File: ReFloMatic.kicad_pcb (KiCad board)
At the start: 2 copper layers, 54.4 x 85.3 mm, 150 parts, among them CON2 MicroSD_Card, P1 PROG, P2 THERMOCOUPLE, P3 DOOR_SERVO, P4 OVEN, P5 USB_B, P6 PWR_CONN, Q1 MMUN2211, Q2 MMUN2111, Q3 MMUN2111, Q4 MMUN2211, U1 STM32F030C, U2 MAX31855KASA

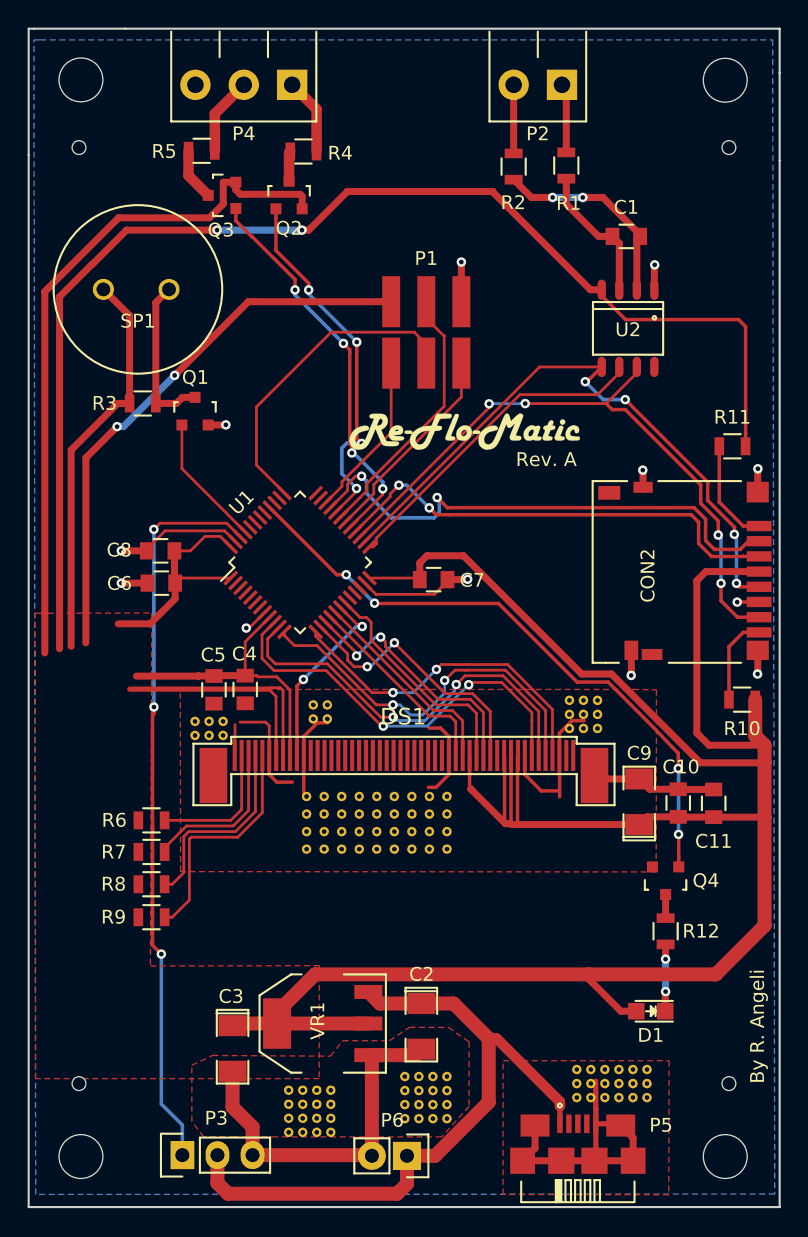
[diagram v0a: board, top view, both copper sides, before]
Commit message: Finished PCB layout. Generated gerbers.
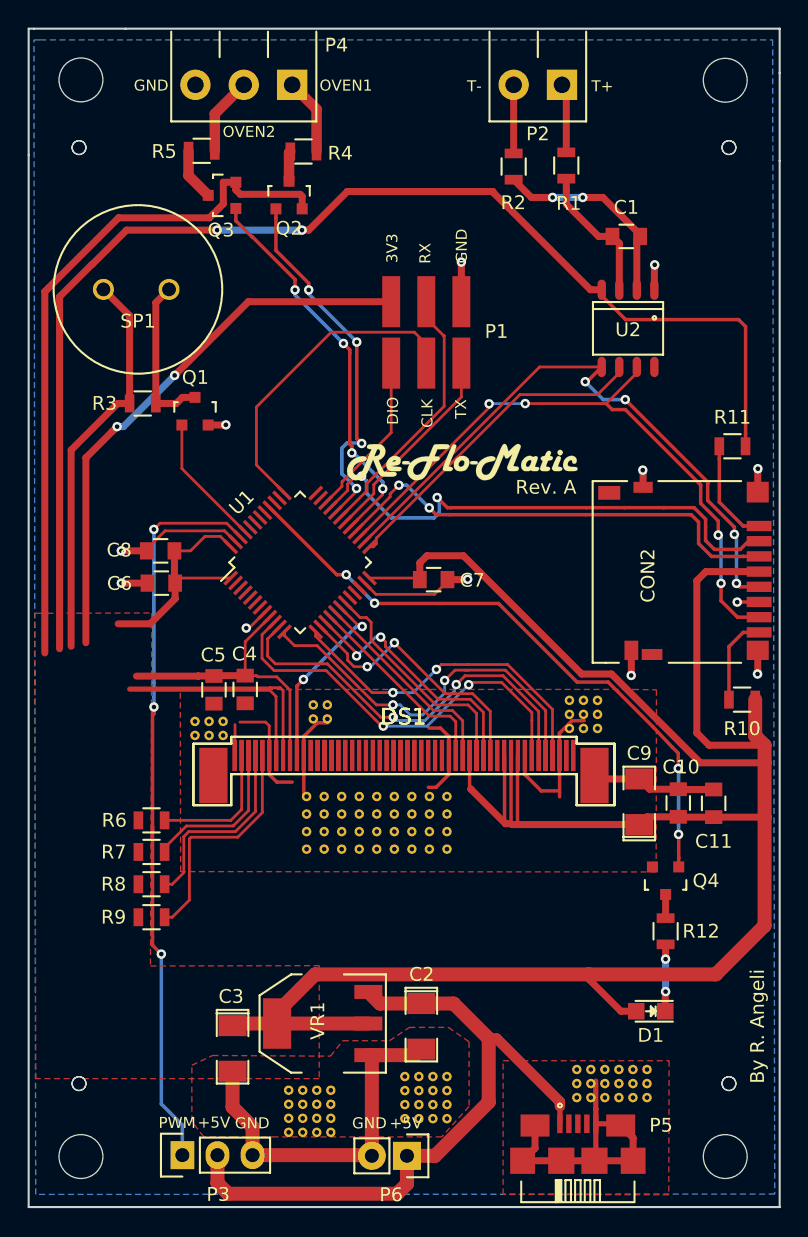
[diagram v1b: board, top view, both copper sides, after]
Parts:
- added DS1: ER-TFT028-4, TFT:ER-TFT028-4, F.Cu at (153.2, 115.7)
- moved G*** 2.22 mm to (157.5, 94.4)
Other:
- board text added: "+5V"
- board text added: "3V3"
- board text added: "CLK"
- board text added: "DIO"
- board text added: "GND"
- board text added: "OVEN1"
- board text added: "OVEN2"
- board text added: "PWM"
- board text added: "RX"
- board text added: "T+"
- board text added: "T-"
- board text added: "TX"
